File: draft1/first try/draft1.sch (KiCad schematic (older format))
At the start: 6 parts, among them IC1 74AVC4TD245PW,118, IC2 74AVC4TD245PW,118, J1 Conn_01x24

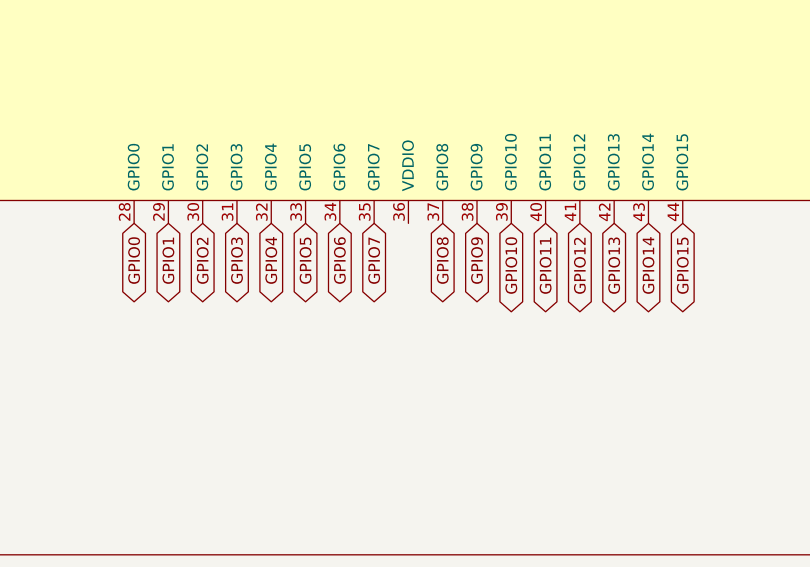
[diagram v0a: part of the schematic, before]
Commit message: added some pins
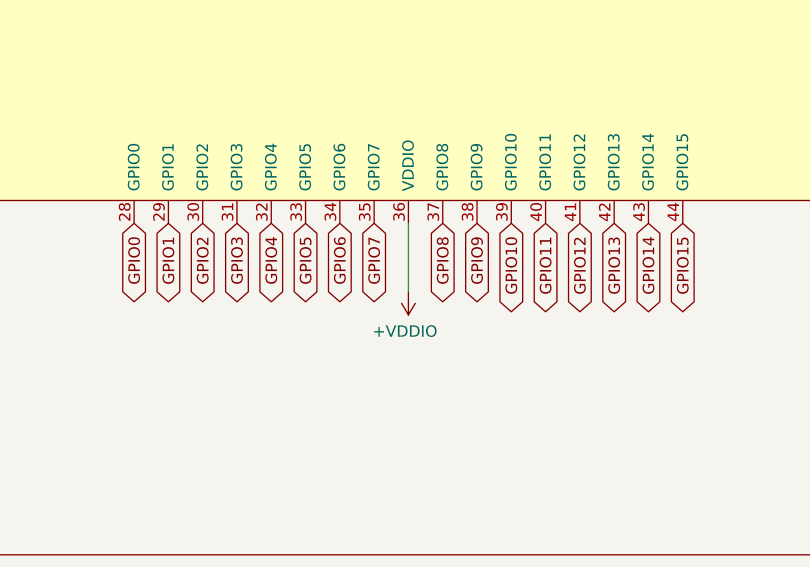
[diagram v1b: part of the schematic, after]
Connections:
- net +VDDIO: now reaches P?.36 (VDDIO)
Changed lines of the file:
@@
 	1    0    0    -1
 $EndComp
+$Comp
+L draft1library:+VDDIO #PWR?
+U 1 1 5F30D677
+P 17800 7350
+F 0 "#PWR?" H 17800 7200 50  0001 C CNN
+F 1 "+VDDIO" H 17815 7523 50  0000 C CNN
+F 2 "" H 17800 7350 50  0001 C CNN
+F 3 "" H 17800 7350 50  0001 C CNN
+	1    17800 7350
+	-1   0    0    1
+$EndComp
+Wire Wire Line
+	17800 7050 17800 7350
 $EndSCHEMATC
